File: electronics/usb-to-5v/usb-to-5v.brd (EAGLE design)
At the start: 10.5 x 15.2 mm, 6 parts

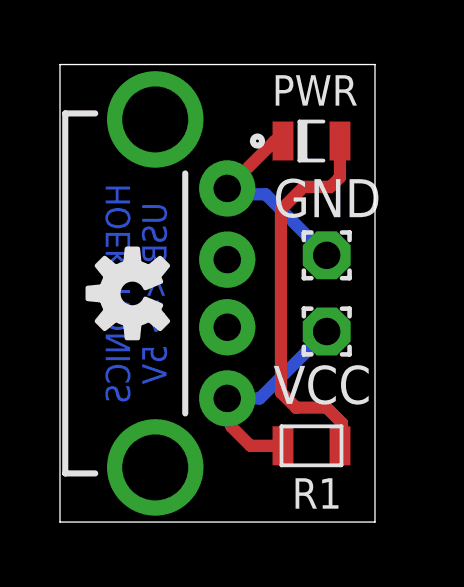
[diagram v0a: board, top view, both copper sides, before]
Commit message: small tweaks to toolpathing stuff.
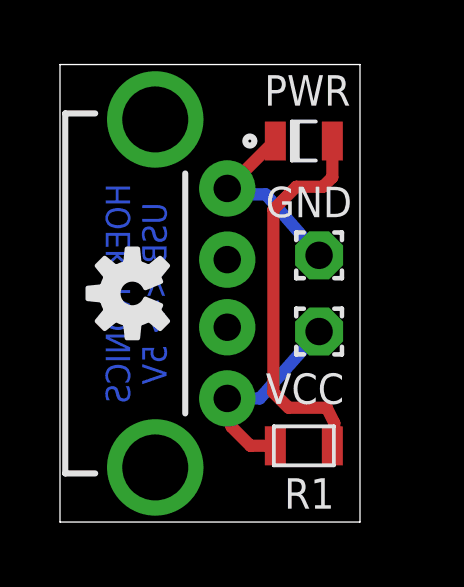
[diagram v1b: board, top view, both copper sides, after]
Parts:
- moved GND 0.25 mm to (8.64, 8.89)
- moved VCC 0.25 mm to (8.64, 6.35)
- moved PWR 0.25 mm to (8.13, 12.7)
- moved R1 0.25 mm to (8.13, 2.54)
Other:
- board size 10.5 x 15.2 mm -> 10 x 15.2 mm
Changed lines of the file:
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@@
 <setting verticaltext="up"/>
 </settings>
-<grid distance="25" unitdist="mil" unit="mil" style="lines" multiple="1" display="yes" altdistance="0.025" altunitdist="inch" altunit="inch"/>
+<grid distance="10" unitdist="mil" unit="mil" style="lines" multiple="1" display="yes" altdistance="0.025" altunitdist="inch" altunit="inch"/>
 <layers>
 <layer number="1" name="Top" color="4" fill="1" visible="yes" active="yes"/>
@@
 <board>
 <plain>
-<wire x1="0" y1="0" x2="10.5" y2="0" width="0" layer="20"/>
-<wire x1="10.5" y1="0" x2="10.5" y2="15.25" width="0" layer="20"/>
-<wire x1="10.5" y1="15.25" x2="0" y2="15.25" width="0" layer="20"/>
+<wire x1="0" y1="0" x2="10" y2="0" width="0" layer="20"/>
+<wire x1="10" y1="0" x2="10" y2="15.25" width="0" layer="20"/>
+<wire x1="10" y1="15.25" x2="0" y2="15.25" width="0" layer="20"/>
 <wire x1="0" y1="15.25" x2="0" y2="0" width="0" layer="20"/>
 <text x="2.54" y="7.62" size="0.8128" layer="16" font="vector" ratio="16" rot="SMR270" align="center">HOEKTRONICS
@@
 <elements>
 <element name="JP1" library="Hoektronics" package="USB-A-H" value="USB-A-H" x="3.175" y="7.62" smashed="yes"/>
-<element name="R1" library="Hoektronics" package="0805-RC" value="1k" x="8.382" y="2.54" smashed="yes" rot="R180">
-<attribute name="NAME" x="9.398" y="1.4605" size="1.016" layer="25" font="vector" rot="R180"/>
+<element name="R1" library="Hoektronics" package="0805-RC" value="1k" x="8.128" y="2.54" smashed="yes" rot="R180">
+<attribute name="NAME" x="9.144" y="1.4605" size="1.016" layer="25" font="vector" rot="R180"/>
 </element>
-<element name="PWR" library="Hoektronics" package="0805-LED" value="" x="8.382" y="12.7" smashed="yes">
-<attribute name="NAME" x="7.066" y="13.8795" size="1.016" layer="25" font="vector"/>
-<attribute name="VALUE" x="7.366" y="11.303" size="0.4064" layer="27"/>
+<element name="PWR" library="Hoektronics" package="0805-LED" value="" x="8.128" y="12.7" smashed="yes">
+<attribute name="NAME" x="6.812" y="13.8795" size="1.016" layer="25" font="vector"/>
+<attribute name="VALUE" x="7.112" y="11.303" size="0.4064" layer="27"/>
 </element>
-<element name="VCC" library="wirepad" package="1,6/0,9" value="" x="8.89" y="6.35" smashed="yes">
-<attribute name="NAME" x="7.112" y="3.937" size="1.27" layer="25" font="vector" ratio="10"/>
-<attribute name="VALUE" x="8.89" y="6.95" size="0.0254" layer="27"/>
+<element name="VCC" library="wirepad" package="1,6/0,9" value="" x="8.636" y="6.35" smashed="yes">
+<attribute name="NAME" x="6.858" y="3.937" size="1.016" layer="25" font="vector" ratio="10"/>
+<attribute name="VALUE" x="8.636" y="6.95" size="0.0254" layer="27"/>
 </element>
-<element name="GND" library="wirepad" package="1,6/0,9" value="" x="8.89" y="8.89" smashed="yes">
-<attribute name="NAME" x="7.112" y="10.16" size="1.27" layer="25" font="vector" ratio="10"/>
-<attribute name="VALUE" x="8.89" y="9.49" size="0.0254" layer="27"/>
+<element name="GND" library="wirepad" package="1,6/0,9" value="" x="8.636" y="8.89" smashed="yes">
+<attribute name="NAME" x="6.858" y="10.16" size="1.016" layer="25" font="vector" ratio="10"/>
+<attribute name="VALUE" x="8.636" y="9.49" size="0.0254" layer="27"/>
 </element>
 <element name="LOGO1" library="SparkFun-Aesthetics" package="OSHW-LOGO-S" value="OSHW-LOGOS" x="2.413" y="7.62" rot="R90"/>
@@
 <contactref element="R1" pad="1"/>
 <contactref element="PWR" pad="A"/>
-<wire x1="9.332" y1="12.7" x2="9.332" y2="11.491" width="0.4064" layer="1"/>
-<wire x1="9.332" y1="11.491" x2="9.017" y2="11.176" width="0.4064" layer="1"/>
-<wire x1="9.017" y1="11.176" x2="8.128" y2="11.176" width="0.4064" layer="1"/>
-<wire x1="8.128" y1="11.176" x2="7.366" y2="10.414" width="0.4064" layer="1"/>
-<wire x1="7.366" y1="10.414" x2="7.366" y2="4.318" width="0.4064" layer="1"/>
-<wire x1="7.366" y1="4.318" x2="7.874" y2="3.81" width="0.4064" layer="1"/>
-<wire x1="7.874" y1="3.81" x2="8.89" y2="3.81" width="0.4064" layer="1"/>
-<wire x1="8.89" y1="3.81" x2="9.398" y2="3.302" width="0.4064" layer="1"/>
-<wire x1="9.398" y1="3.302" x2="9.398" y2="2.728" width="0.4064" layer="1"/>
-<wire x1="9.398" y1="2.728" x2="9.332" y2="2.54" width="0.4064" layer="1"/>
+<wire x1="9.078" y1="12.7" x2="9.078" y2="11.491" width="0.4064" layer="1"/>
+<wire x1="9.078" y1="11.491" x2="8.763" y2="11.176" width="0.4064" layer="1"/>
+<wire x1="8.763" y1="11.176" x2="7.874" y2="11.176" width="0.4064" layer="1"/>
+<wire x1="7.874" y1="11.176" x2="7.112" y2="10.414" width="0.4064" layer="1"/>
+<wire x1="7.112" y1="10.414" x2="7.112" y2="4.318" width="0.4064" layer="1"/>
+<wire x1="7.112" y1="4.318" x2="7.62" y2="3.81" width="0.4064" layer="1"/>
+<wire x1="7.62" y1="3.81" x2="8.89" y2="3.81" width="0.4064" layer="1"/>
+<wire x1="8.89" y1="3.81" x2="9.144" y2="3.302" width="0.4064" layer="1"/>
+<wire x1="9.144" y1="3.302" x2="9.144" y2="2.728" width="0.4064" layer="1"/>
+<wire x1="9.144" y1="2.728" x2="9.078" y2="2.54" width="0.4064" layer="1"/>
 </signal>
 <signal name="VCC">
@@
 <contactref element="R1" pad="2"/>
 <contactref element="VCC" pad="1"/>
-<wire x1="7.432" y1="2.54" x2="6.35" y2="2.54" width="0.4064" layer="1"/>
+<wire x1="7.178" y1="2.54" x2="6.35" y2="2.54" width="0.4064" layer="1"/>
 <wire x1="6.35" y1="2.54" x2="5.715" y2="3.175" width="0.4064" layer="1"/>
 <wire x1="5.715" y1="3.175" x2="5.715" y2="3.98" width="0.4064" layer="1"/>
 <wire x1="5.715" y1="3.98" x2="5.575" y2="4.12" width="0.4064" layer="1"/>
 <wire x1="5.575" y1="4.12" x2="6.66" y2="4.12" width="0.4064" layer="16"/>
-<wire x1="6.66" y1="4.12" x2="8.89" y2="6.35" width="0.4064" layer="16"/>
+<wire x1="6.66" y1="4.12" x2="8.636" y2="6.35" width="0.4064" layer="16"/>
 </signal>
 <signal name="GND">
@@
 <contactref element="PWR" pad="C"/>
 <contactref element="GND" pad="1"/>
-<wire x1="8.89" y1="8.89" x2="6.858" y2="10.922" width="0.4064" layer="16"/>
+<wire x1="8.636" y1="8.89" x2="6.858" y2="10.922" width="0.4064" layer="16"/>
 <wire x1="6.858" y1="10.922" x2="5.773" y2="10.922" width="0.4064" layer="16"/>
 <wire x1="5.773" y1="10.922" x2="5.575" y2="11.12" width="0.4064" layer="16"/>
-<wire x1="7.432" y1="12.7" x2="7.155" y2="12.7" width="0.4064" layer="1"/>
+<wire x1="7.178" y1="12.7" x2="7.155" y2="12.7" width="0.4064" layer="1"/>
 <wire x1="7.155" y1="12.7" x2="5.575" y2="11.12" width="0.4064" layer="1"/>
 </signal>
